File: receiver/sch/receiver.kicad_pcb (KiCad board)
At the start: 2 copper layers, 45 x 58 mm, 21 parts, among them CON1 AVR-ISP-6, IC1 ATTINY85-S, P1 MOTOR, P2 MAIN_BUTTON, P3 MX-05V, P4 LEDs, Q1 S8050, Q2 S8550, Q3 S8550, Q4 S8050, Q5 2N7002, Q6 2N7002

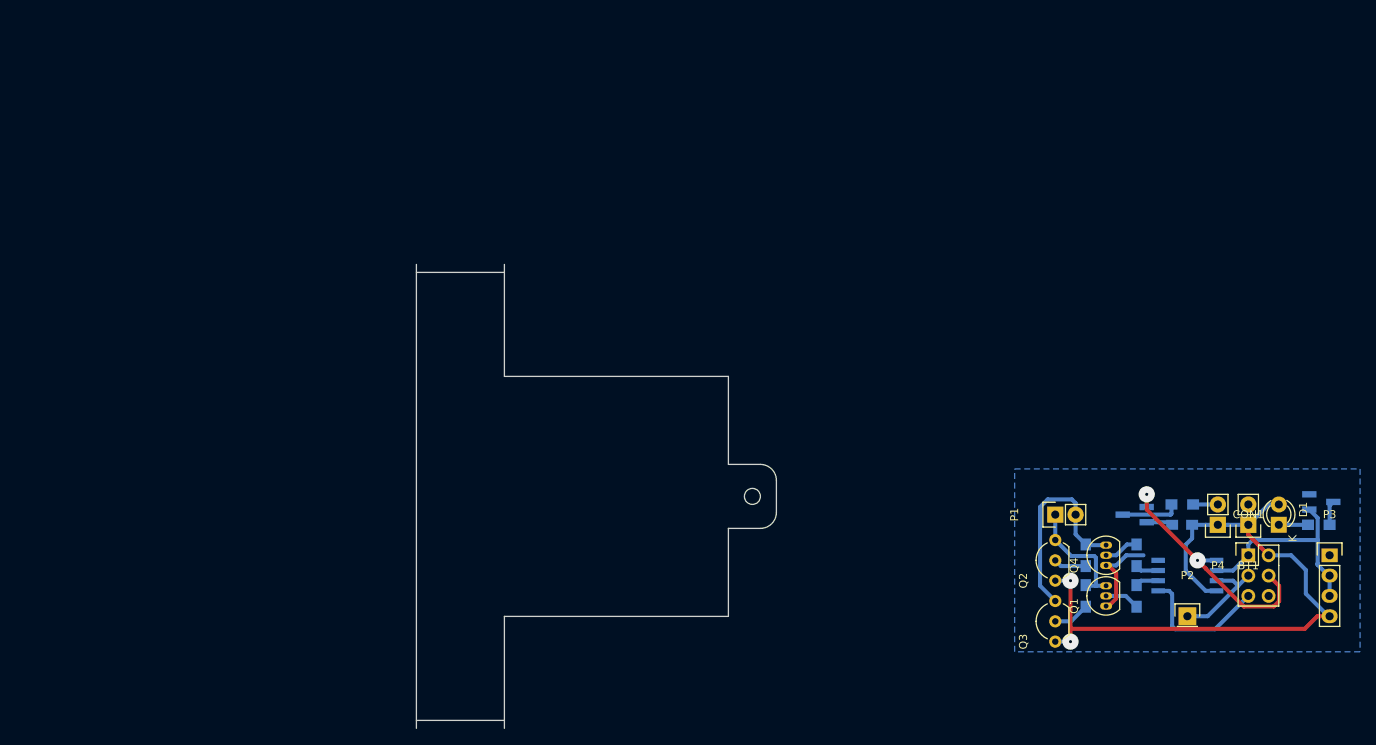
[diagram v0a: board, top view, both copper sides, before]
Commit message: receiver board layout update
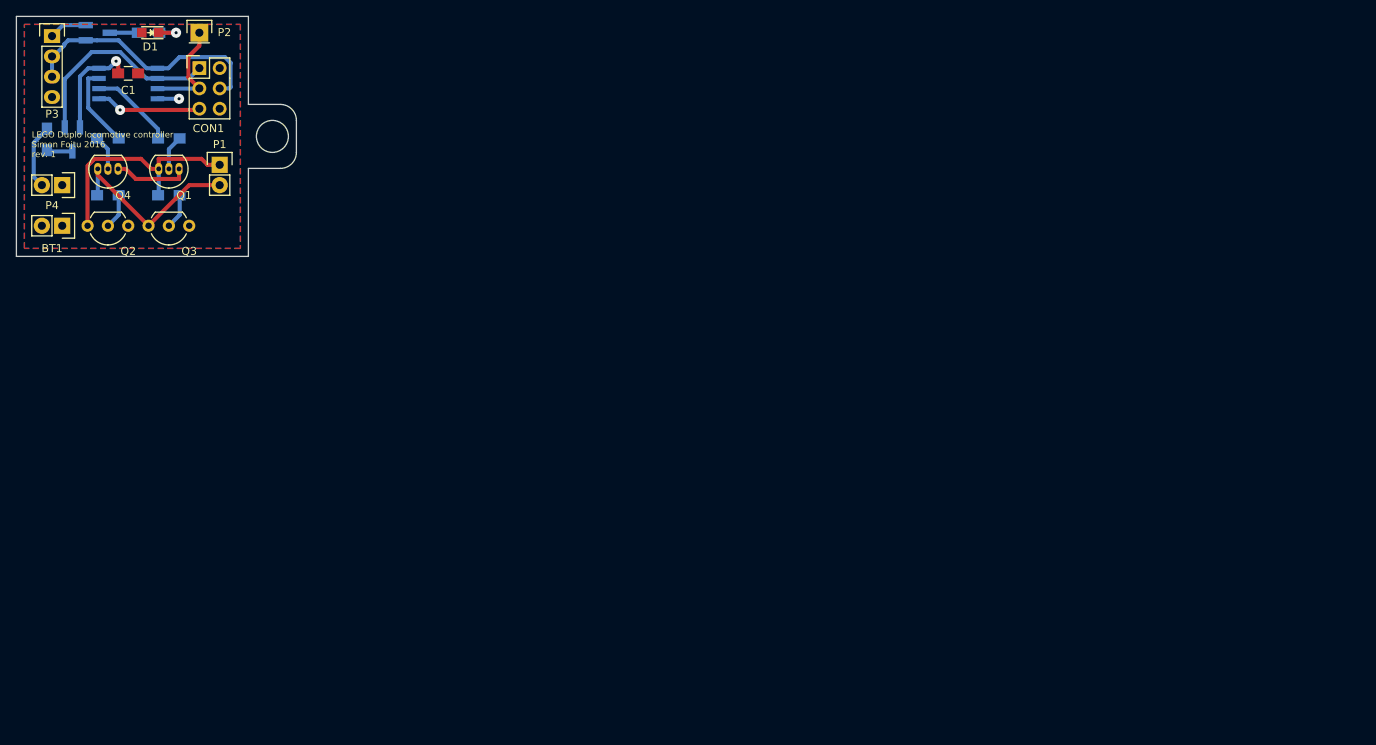
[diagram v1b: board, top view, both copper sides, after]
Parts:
- C1: moved to F.Cu
- D1: value red -> RX; footprint LEDs:LED-3MM -> LEDs:LED_0805
- P2: value MAIN_BUTTON -> MAIN_BTN
- moved P3 172.4 mm to (24.5, 21.5)
- moved Q5 163.8 mm to (30.2, 21.0)
- moved R5 158.7 mm to (36.5, 21.0), turned to 180 degrees
- moved D1 153.9 mm to (36.7, 21.0), turned to 180 degrees
- moved BT1 152.9 mm to (25.7, 45.2), turned to 270 degrees
- moved P4 150.6 mm to (25.7, 40.1), turned to 270 degrees
- moved R6 149.1 mm to (23.8, 34.4), turned to 270 degrees
- moved IC1 146.0 mm to (34.0, 27.4)
- moved CON1 144.6 mm to (42.9, 25.5)
- moved P2 143.4 mm to (42.9, 21.0)
- moved C1 143.3 mm to (34.0, 26.1)
- moved Q6 140.8 mm to (27.0, 34.4), turned to 0 degrees
- moved R4 138.7 mm to (31.4, 34.2), turned to 180 degrees
- moved R1 133.8 mm to (39.1, 34.2), turned to 180 degrees
- moved Q4 133.1 mm to (32.7, 38.1), turned to 180 degrees
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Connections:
- CON1 pad 1: /MISO -> /MCU-LED
- CON1 pad 4: /MCU-LED -> /MOSI
- IC1 pad 5: /MCU-LED -> /MOSI
- IC1 pad 6: /MISO -> /MCU-LED
- P3 pad 2: /MISO -> /MOSI
- P3 pad 3: /MISO -> /MOSI
- Q5 pad 1: /MISO -> /MOSI
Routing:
- net +5V: track 85.1 -> 2.70 mm, vias 2 -> 1
- net /MOSI: track 0.00 -> 32.6 mm
- net /MISO: track 27.0 -> 0.00 mm
- net Net-(P1-Pad1): track 15.2 -> 29.8 mm
- net GND: track 16.0 -> 27.5 mm, vias 0 -> 1
- net /MOT_A: track 2.93 -> 10.6 mm
- net /MOT_B: track 2.93 -> 10.4 mm
- net /MCU-LED: track 31.5 -> 26.2 mm, vias 2 -> 0
- net Net-(P4-Pad2): track 3.09 -> 8.17 mm
- net /RST: track 17.3 -> 13.2 mm, vias 0 -> 1
- net Net-(Q6-Pad3): track 7.30 -> 3.24 mm
- net Net-(P1-Pad2): track 25.9 -> 24.1 mm
- net /MAIN_BUTTON: track 12.7 -> 13.3 mm
- net Net-(D1-Pad1): track 3.65 -> 4.26 mm, vias 0 -> 1
- added copper zone on F.Cu, net +5V
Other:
- board size 45 x 58 mm -> 35 x 30 mm
- net class Default: clearance 0.2032 -> 0.254; via_dia 2.032 -> 1.27
- rule trace_clearance: 0.2032 -> 0.254
- rule trace_min: 0.2 -> 0.254
- rule via_min_size: 0.4 -> 1.016
- board text added: "LEGO Duplo locomotive controller Simon Fojtu 2016 rev. 1"
